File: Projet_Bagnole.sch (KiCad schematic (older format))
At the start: 50 parts, among them J1 USB_A, J2 Conn_01x03_Male, J3 Conn_01x04_Male, J4 AVR-ISP-6, M1 Motor_DC, M2 Stepper_Motor_bipolar, U1 ATmega16U2-AU, U2 DRV8210DRL, U3 MAX1811, Y1 Crystal_GND24

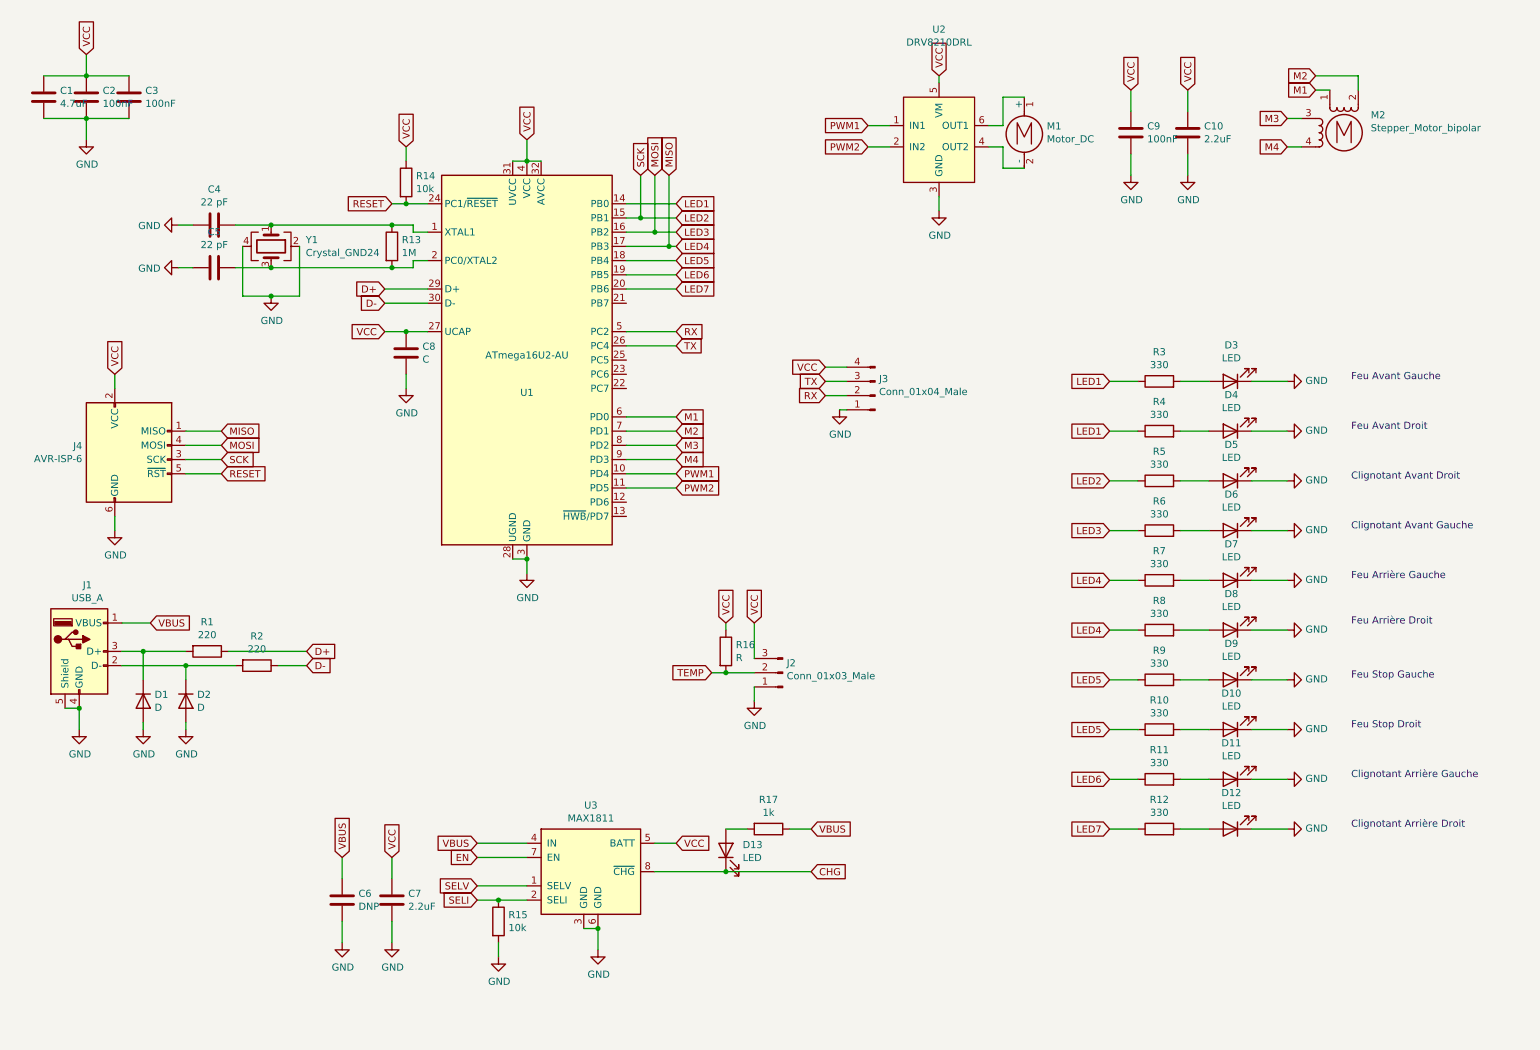
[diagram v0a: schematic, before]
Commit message: V2
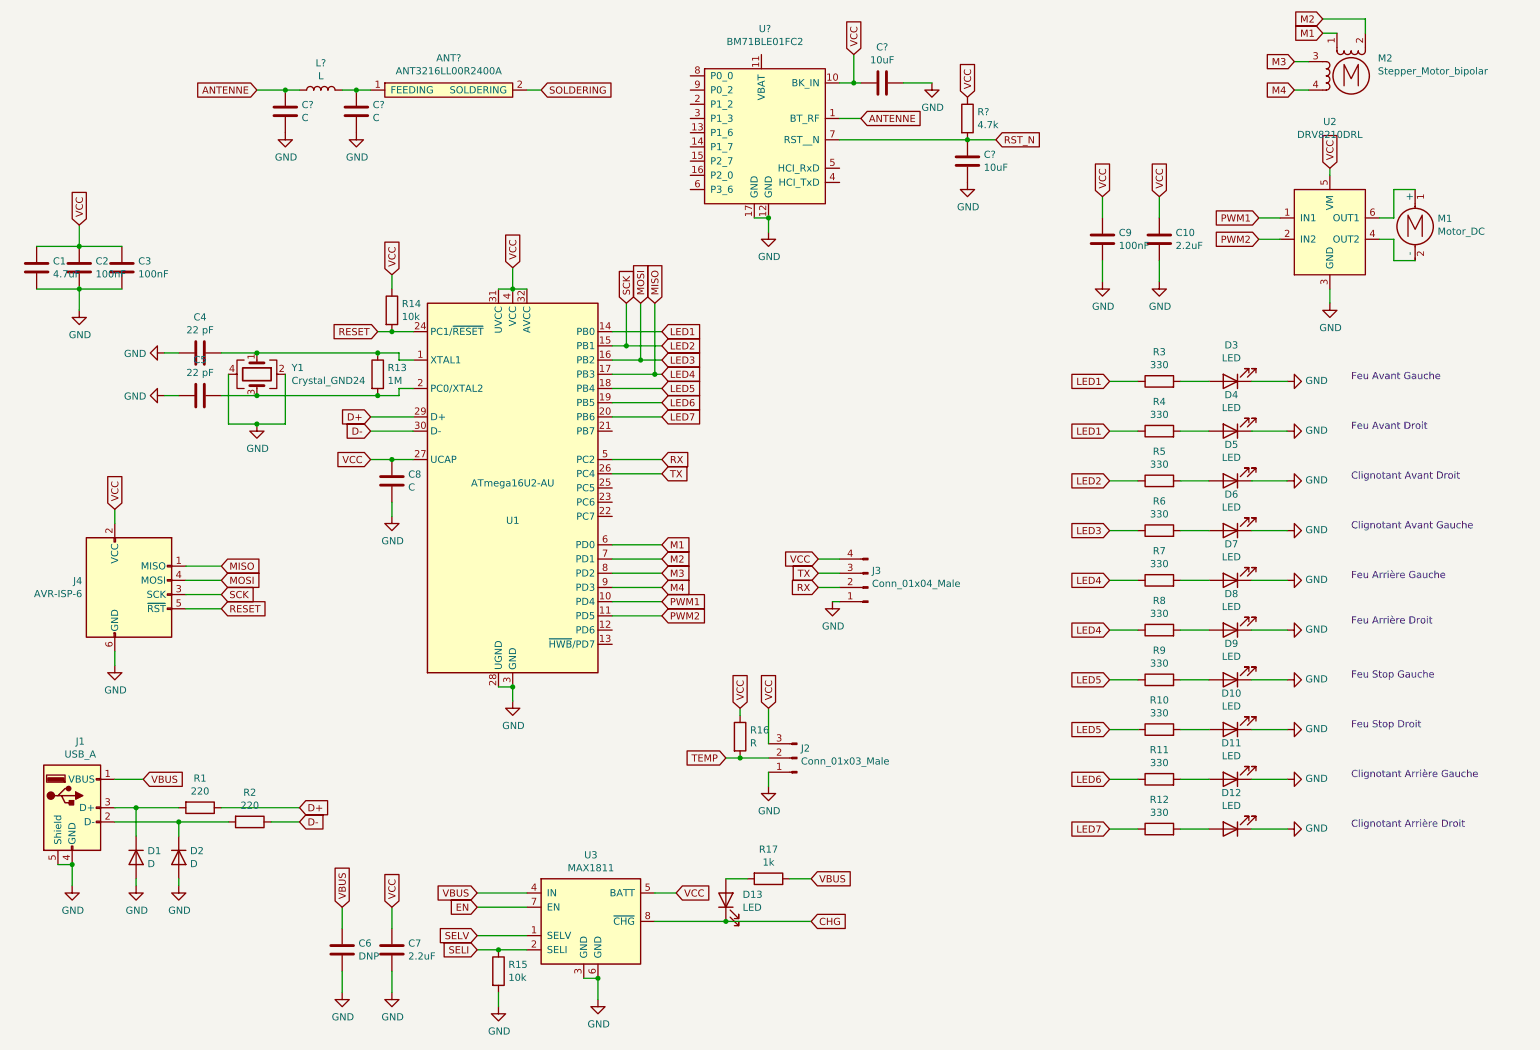
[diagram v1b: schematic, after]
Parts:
- added ANT?: ANT3216LL00R2400A, symbol Projet_Bagnole-rescue:ANT3216LL00R2400A
- added C? (x2): C, symbol Device:C
- added C? (x2): 10uF, symbol Device:C
- added L?: L, symbol Device:L
- added R?: 4.7k, symbol Device:R
- added U?: BM71BLE01FC2, symbol Projet_Bagnole-rescue:BM71BLE01FC2
- M1: footprint (none) -> Connector_PinHeader_2.54mm:PinHeader_1x02_P2.54mm_Vertical
- M2: footprint (none) -> Connector_PinHeader_2.54mm:PinHeader_2x02_P2.54mm_Vertical
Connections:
- net GND: now also C?.1, C?.2, C?.2, C?.2, U?.12 (GND), U?.17 (GND)
- net VCC: now also C?.2, R?.1, U?.10 (BK_IN)
- new net: ANT?.1 (FEEDING), C?.1, L?.2
- new net ANTENNE: C?.1, L?.1, U?.1 (BT_RF)
- new net RST_N: C?.1, R?.2, U?.7 (RST__N)
- new net SOLDERING: ANT?.2 (SOLDERING)
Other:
- moved on the sheet: C1, C10, C2, C3, C4, C5, C6, C7, C8, C9, D1, D13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
